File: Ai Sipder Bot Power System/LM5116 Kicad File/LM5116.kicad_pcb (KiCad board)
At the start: 4 copper layers, 60.2 x 83.5 mm, 89 parts, among them J1 XT60-M, J10 PH1-01-UA, J11 PH1-01-UA, J12 PH1-01-UA, J13 PH1-01-UA, J14 61300311121, J15 61300311121, J16 61300311121, J17 61300311121, J18 61300311121, J19 61300311121, J2 PH1-01-UA, J20 61300311121, J21 61300311121, J22 61300311121, J23 61300311121, J24 61300311121, J25 61300311121, J26 691137710002, J3 PH1-01-UA, J4 PH1-01-UA, J5 PH1-01-UA, J6 PH1-01-UA, J7 PH1-01-UA, J8 PH1-01-UA, J9 PH1-01-UA, Q1 CSD17304Q3, Q2 CSD17304Q3, Q3 CSD17304Q3, Q4 CSD17304Q3, Q5 2N7002, Q6 IQDH29NE2LM5CG, U1 LM25116MHX/NOPB, U2 TLV1701AIDBVR, U3 TL431DBZ

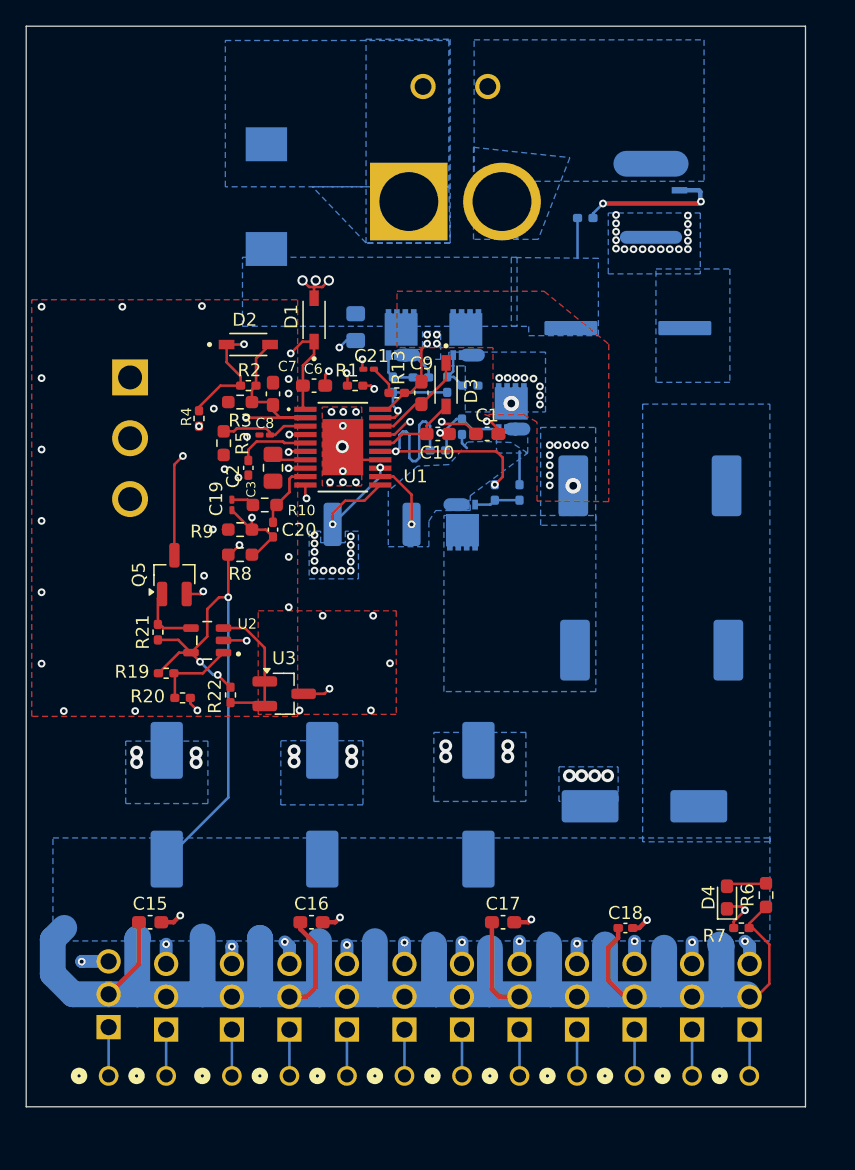
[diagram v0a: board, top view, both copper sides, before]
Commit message: Adjust Kicad File
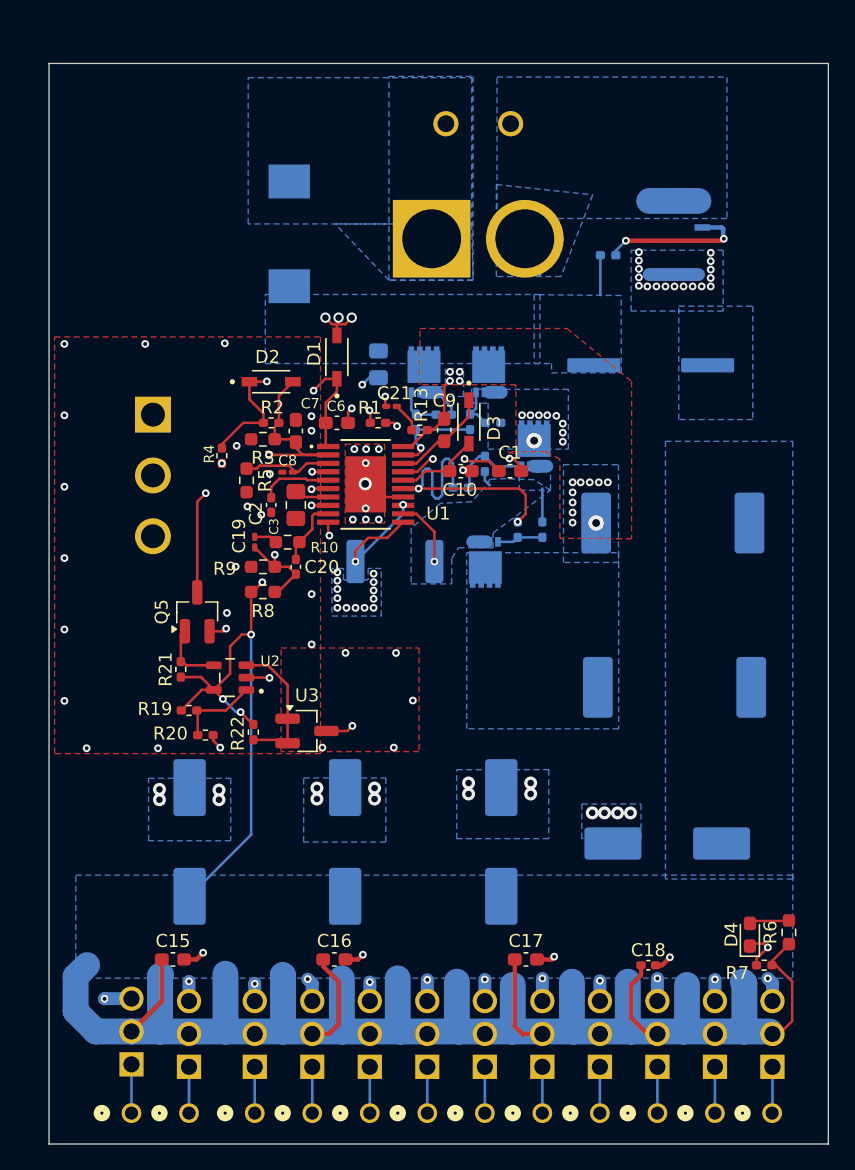
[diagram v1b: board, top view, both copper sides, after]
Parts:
- moved J1 3.37 mm to (146.1, 64.5)
- moved C8 3.37 mm to (131.3, 82.6)
- moved C9 3.37 mm to (143.4, 79.3)
- moved D3 3.37 mm to (145.3, 78.7)
- moved D4 3.37 mm to (167.0, 118.3)
- moved J11 3.37 mm to (133.2, 132.1)
- moved J12 3.37 mm to (137.7, 132.1)
- moved J17 3.37 mm to (155.4, 126.0)
- moved J21 3.37 mm to (137.7, 126.0)
- moved J22 3.37 mm to (133.2, 126.0)
- moved J26 3.37 mm to (146.1, 55.6)
- moved J5 3.37 mm to (155.4, 132.1)
- moved Q1 3.37 mm to (146.9, 74.9)
- moved R10 3.37 mm to (131.3, 88.0)
- moved R12 3.37 mm to (141.2, 78.7)
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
